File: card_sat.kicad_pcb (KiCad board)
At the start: 2 copper layers, 115 x 127 mm, 20 parts, among them J1 Conn_01x05_Male, J2 Conn_01x05_Male, J3 Conn_01x05_Male, J4 Conn_01x05_Male, J5 Conn_01x04_Male, U1 Pico

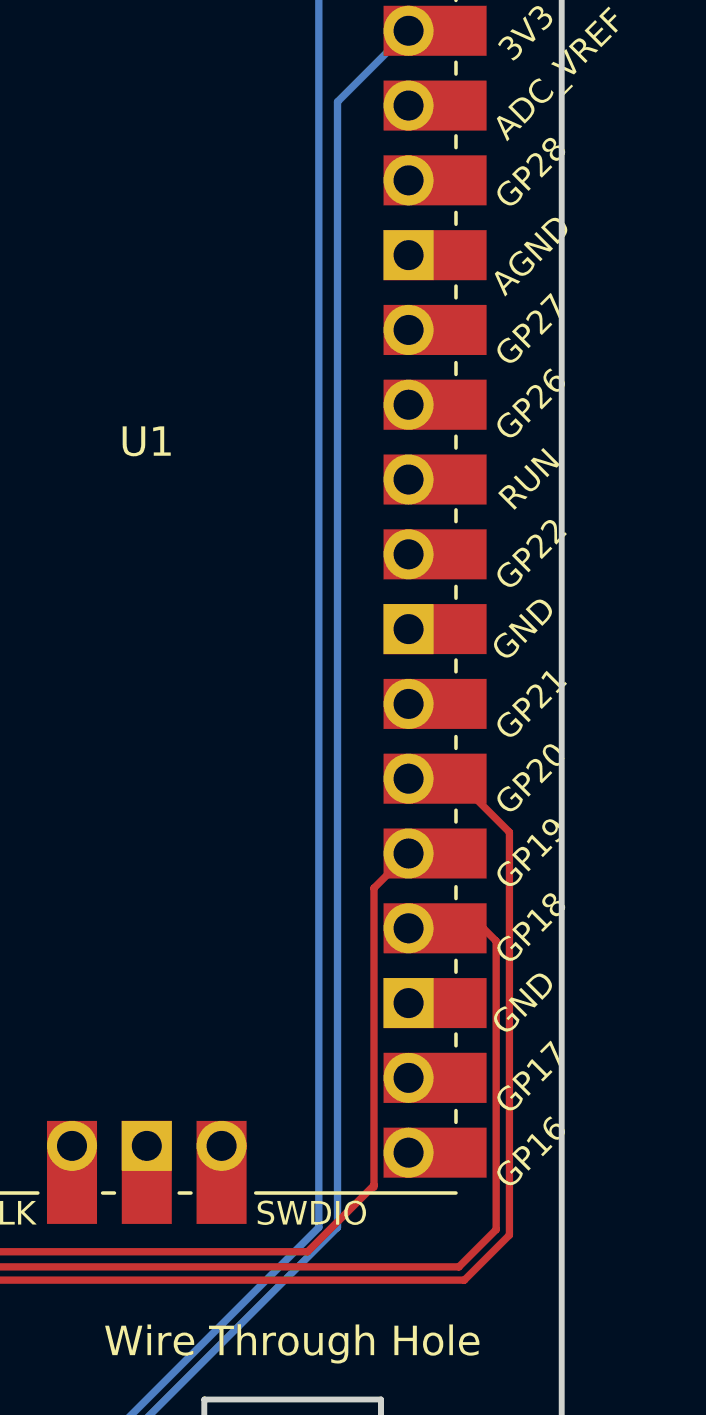
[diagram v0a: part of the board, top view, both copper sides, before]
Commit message: debugging still :(
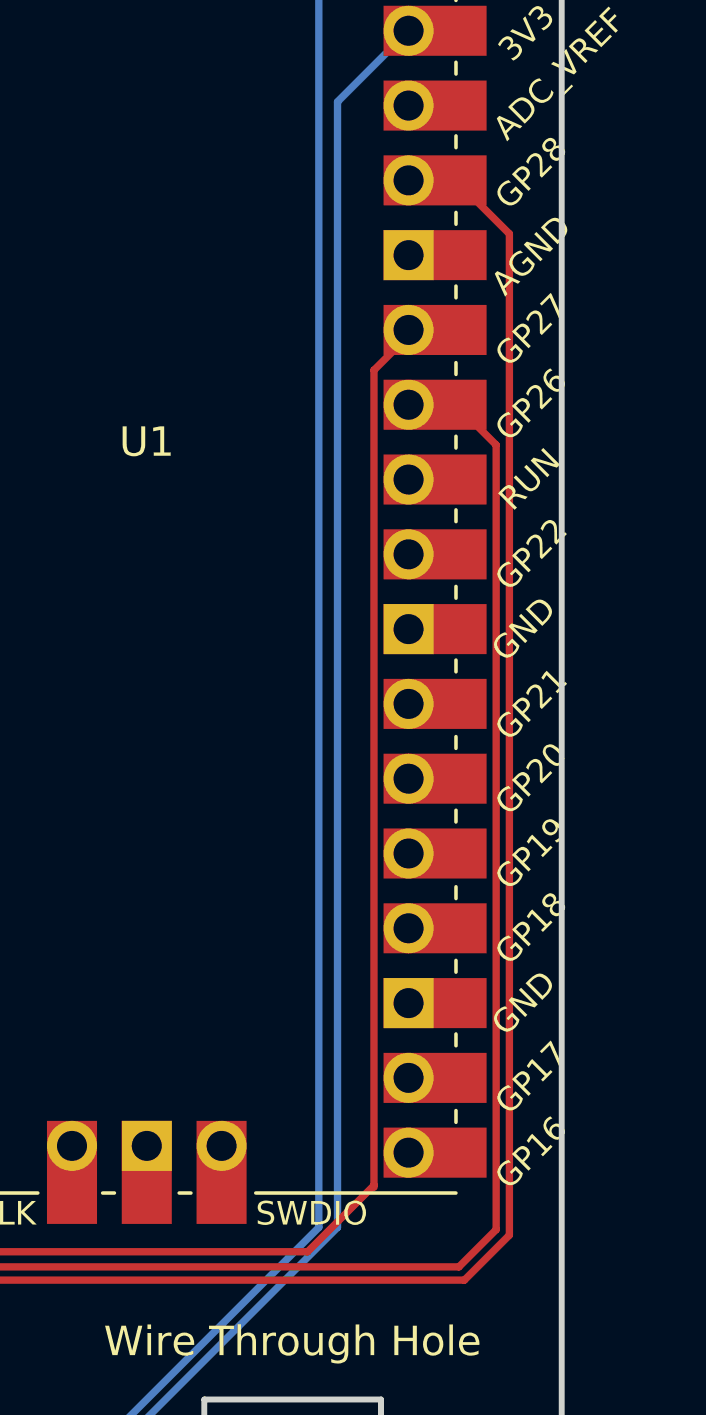
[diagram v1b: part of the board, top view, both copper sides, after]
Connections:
- U1 pad 24: Net-(R4-Pad2) -> unconnected-(U1-Pad24)
- U1 pad 25: Net-(R5-Pad2) -> unconnected-(U1-Pad25)
- U1 pad 26: Net-(R8-Pad2) -> unconnected-(U1-Pad26)
- U1 pad 31: unconnected-(U1-Pad31) -> Net-(R4-Pad2)
- U1 pad 32: unconnected-(U1-Pad32) -> Net-(R5-Pad2)
- U1 pad 34: unconnected-(U1-Pad34) -> Net-(R8-Pad2)
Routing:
- net Net-(R8-Pad2): track 81.7 -> 102.0 mm
- net Net-(R4-Pad2): track 68.7 -> 86.0 mm
- net Net-(R5-Pad2): track 64.2 -> 79.9 mm
- net unconnected-(U1-Pad25): track 0.00 -> 2.09 mm
- net unconnected-(U1-Pad26): track 0.00 -> 1.61 mm
